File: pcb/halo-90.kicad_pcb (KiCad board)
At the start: 4 copper layers, 23.4 x 23.3 mm, 101 parts, among them U1 STM8L151G6

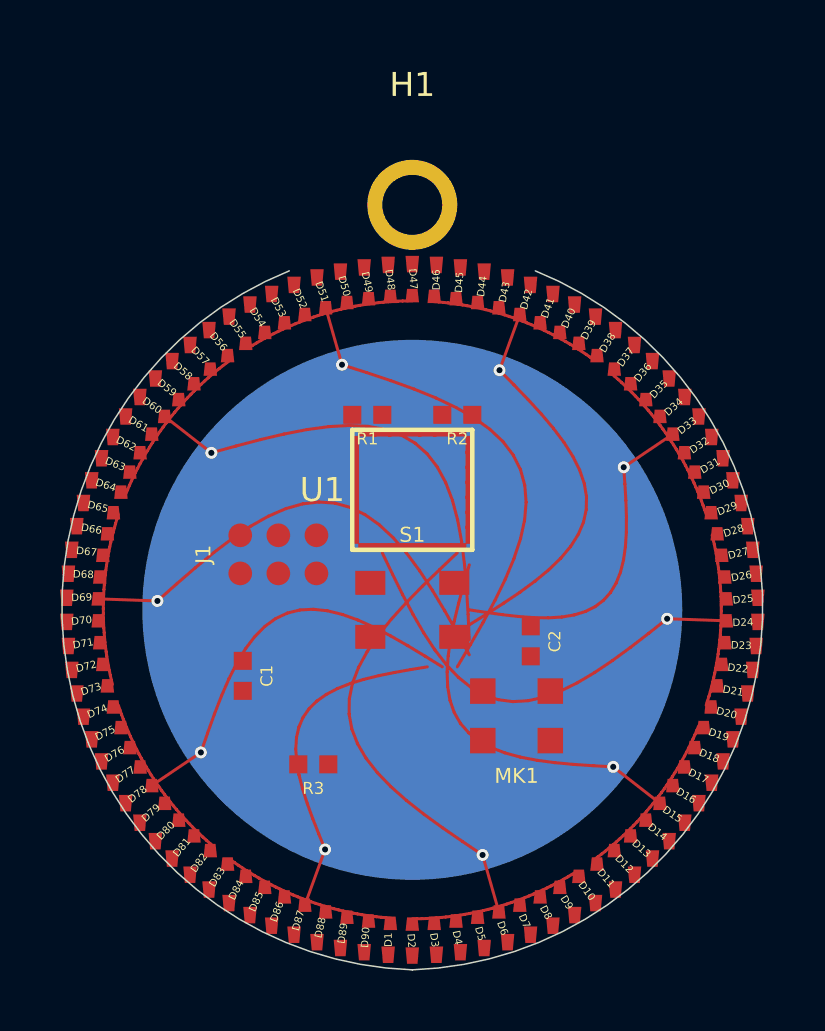
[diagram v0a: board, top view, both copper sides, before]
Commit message: To explore later, current save
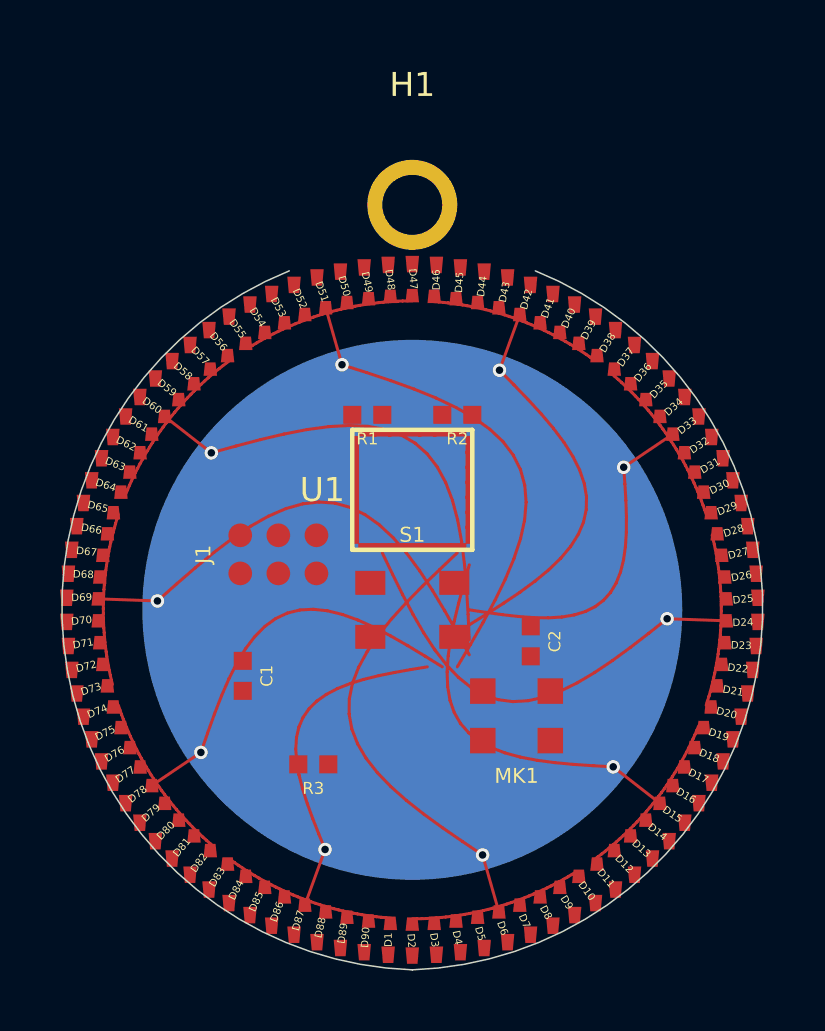
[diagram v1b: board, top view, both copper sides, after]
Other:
- net class Default: via_dia 0.4 -> 0.45; via_drill 0.2 -> 0.25
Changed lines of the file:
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@@
     (clearance 0.1)
     (trace_width 0.1)
-    (via_dia 0.4)
-    (via_drill 0.2)
+    (via_dia 0.45)
+    (via_drill 0.25)
   )
 (module STM8L15xxx:UFQFPN28 (layer "Front") (at 0 -4 90)
@@
 (segment (start 5.1846 8.9) (end 5.322 8.8185) (width 0.1) (layer "Front")  (net 3))
 (segment (start 5.322 8.8185) (end 5.4582 8.7349) (width 0.1) (layer "Front")  (net 3))
-(via (at 2.342917524444493 8.17072441547571) (size 0.4) (drill 0.2) (layers "Front" "Back")  (net 3))
+(via (at 2.342917524444493 8.17072441547571) (size 0.45) (drill 0.25) (layers "Front" "Back")  (net 3))
 (segment (start 1.5 -1.9) (end 0.9119825216212106 -1.3437192384224104) (width 0.1) (layer "Front")  (net 3))
 (segment (start 0.9119825216212106 -1.3437192384224104) (end 0.3394817564249679 -0.7887372224885054) (width 0.1) (layer "Front")  (net 3))
@@
 (segment (start 9.4257 4.1529) (end 9.489 4.0061) (width 0.1) (layer "Front")  (net 4))
 (segment (start 9.489 4.0061) (end 9.55 3.8584) (width 0.1) (layer "Front")  (net 4))
-(via (at 6.698091405657137 5.233122540268096) (size 0.4) (drill 0.2) (layers "Front" "Back")  (net 4))
+(via (at 6.698091405657137 5.233122540268096) (size 0.45) (drill 0.25) (layers "Front" "Back")  (net 4))
 (segment (start 1.9 -1.5) (end 1.718587601227993 -0.8631091280833536) (width 0.1) (layer "Front")  (net 4))
 (segment (start 1.718587601227993 -0.8631091280833536) (end 1.5475494245049704 -0.23361103200821653) (width 0.1) (layer "Front")  (net 4))
@@
 (segment (start 10.0665 -2.1805) (end 10.0315 -2.3365) (width 0.1) (layer "Front")  (net 5))
 (segment (start 10.0315 -2.3365) (end 9.994 -2.4918) (width 0.1) (layer "Front")  (net 5))
-(via (at 8.494822029662314 0.29664572197125916) (size 0.4) (drill 0.2) (layers "Front" "Back")  (net 5))
+(via (at 8.494822029662314 0.29664572197125916) (size 0.45) (drill 0.25) (layers "Front" "Back")  (net 5))
 (segment (start -1 -1.9) (end -0.6627113378766785 -1.1960407519564675) (width 0.1) (layer "Front")  (net 5))
 (segment (start -0.6627113378766785 -1.1960407519564675) (end -0.3220381405178265 -0.5067108815103598) (width 0.1) (layer "Front")  (net 5))
@@
 (segment (start 6.8623 -7.6811) (end 6.7423 -7.7866) (width 0.1) (layer "Front")  (net 6))
 (segment (start 6.7423 -7.7866) (end 6.6207 -7.8903) (width 0.1) (layer "Front")  (net 6))
-(via (at 7.0468193667178545 -4.753139679501347) (size 0.4) (drill 0.2) (layers "Front" "Back")  (net 6))
+(via (at 7.0468193667178545 -4.753139679501347) (size 0.45) (drill 0.25) (layers "Front" "Back")  (net 6))
 (segment (start 1.9 0) (end 2.4547629135456077 0.08439898974141563) (width 0.1) (layer "Front")  (net 6))
 (segment (start 2.4547629135456077 0.08439898974141563) (end 3.002202311713308 0.16086789256743395) (width 0.1) (layer "Front")  (net 6))
@@
 (segment (start 1.0369 -10.2477) (end 0.8778 -10.2625) (width 0.1) (layer "Front")  (net 7))
 (segment (start 0.8778 -10.2625) (end 0.7185 -10.2749) (width 0.1) (layer "Front")  (net 7))
-(via (at 2.9071712182681857 -7.987387276680221) (size 0.4) (drill 0.2) (layers "Front" "Back")  (net 7))
+(via (at 2.9071712182681857 -7.987387276680221) (size 0.45) (drill 0.25) (layers "Front" "Back")  (net 7))
 (segment (start 1.9 0.5) (end 2.4814465162001023 0.1386531524594694) (width 0.1) (layer "Front")  (net 7))
 (segment (start 2.4814465162001023 0.1386531524594694) (end 3.0498158843611756 -0.22424551859194658) (width 0.1) (layer "Front")  (net 7))
@@
 (segment (start -5.1846 -8.9) (end -5.322 -8.8185) (width 0.1) (layer "Front")  (net 8))
 (segment (start -5.322 -8.8185) (end -5.4582 -8.7349) (width 0.1) (layer "Front")  (net 8))
-(via (at -2.3429175244444913 -8.17072441547571) (size 0.4) (drill 0.2) (layers "Front" "Back")  (net 8))
+(via (at -2.3429175244444913 -8.17072441547571) (size 0.45) (drill 0.25) (layers "Front" "Back")  (net 8))
 (segment (start 1.5 1.9) (end 1.938017478378789 1.1559978803741333) (width 0.1) (layer "Front")  (net 8))
 (segment (start 1.938017478378789 1.1559978803741333) (end 2.360518243575032 0.4179168292385686) (width 0.1) (layer "Front")  (net 8))
@@
 (segment (start -9.4257 -4.1529) (end -9.489 -4.0061) (width 0.1) (layer "Front")  (net 9))
 (segment (start -9.489 -4.0061) (end -9.55 -3.8584) (width 0.1) (layer "Front")  (net 9))
-(via (at -6.698091405657138 -5.233122540268093) (size 0.4) (drill 0.2) (layers "Front" "Back")  (net 9))
+(via (at -6.698091405657138 -5.233122540268093) (size 0.45) (drill 0.25) (layers "Front" "Back")  (net 9))
 (segment (start 1.9 1) (end 1.8601255057639607 0.15032874122220274) (width 0.1) (layer "Front")  (net 9))
 (segment (start 1.8601255057639607 0.15032874122220274) (end 1.8106471766200398 -0.6860947994417036) (width 0.1) (layer "Front")  (net 9))
@@
 (segment (start -10.0665 2.1805) (end -10.0315 2.3365) (width 0.1) (layer "Front")  (net 10))
 (segment (start -10.0315 2.3365) (end -9.994 2.4918) (width 0.1) (layer "Front")  (net 10))
-(via (at -8.494822029662313 -0.29664572197126404) (size 0.4) (drill 0.2) (layers "Front" "Back")  (net 10))
+(via (at -8.494822029662313 -0.29664572197126404) (size 0.45) (drill 0.25) (layers "Front" "Back")  (net 10))
 (segment (start 1.9 1.5) (end 1.492681823470242 0.7597243445419842) (width 0.1) (layer "Front")  (net 10))
 (segment (start 1.492681823470242 0.7597243445419842) (end 1.0825954214178357 0.035464763535378196) (width 0.1) (layer "Front")  (net 10))
@@
 (segment (start -6.8623 7.6811) (end -6.7423 7.7866) (width 0.1) (layer "Front")  (net 11))
 (segment (start -6.7423 7.7866) (end -6.6207 7.8903) (width 0.1) (layer "Front")  (net 11))
-(via (at -7.046819366717857 4.753139679501343) (size 0.4) (drill 0.2) (layers "Front" "Back")  (net 11))
+(via (at -7.046819366717857 4.753139679501343) (size 0.45) (drill 0.25) (layers "Front" "Back")  (net 11))
 (segment (start 1 1.9) (end 0.4191272798849677 1.5391370308119163) (width 0.1) (layer "Front")  (net 11))
 (segment (start 0.4191272798849677 1.5391370308119163) (end -0.15734939598834818 1.1906723939576263) (width 0.1) (layer "Front")  (net 11))
@@
 (segment (start -1.0369 10.2477) (end -0.8778 10.2625) (width 0.1) (layer "Front")  (net 12))
 (segment (start -0.8778 10.2625) (end -0.7185 10.2749) (width 0.1) (layer "Front")  (net 12))
-(via (at -2.907171218268183 7.987387276680222) (size 0.4) (drill 0.2) (layers "Front" "Back")  (net 12))
+(via (at -2.907171218268183 7.987387276680222) (size 0.45) (drill 0.25) (layers "Front" "Back")  (net 12))
 (segment (start 0.5 1.9) (end -0.05126942976148058 1.9911697611019092) (width 0.1) (layer "Front")  (net 12))
 (segment (start -0.05126942976148058 1.9911697611019092) (end -0.5931595697612257 2.0875892039919974) (width 0.1) (layer "Front")  (net 12))
